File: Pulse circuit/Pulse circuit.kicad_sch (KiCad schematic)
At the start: 5 parts, among them U1 module_max30102, U2 module_max30102, U3 DOIT-ESP32-DEVKIT-V1

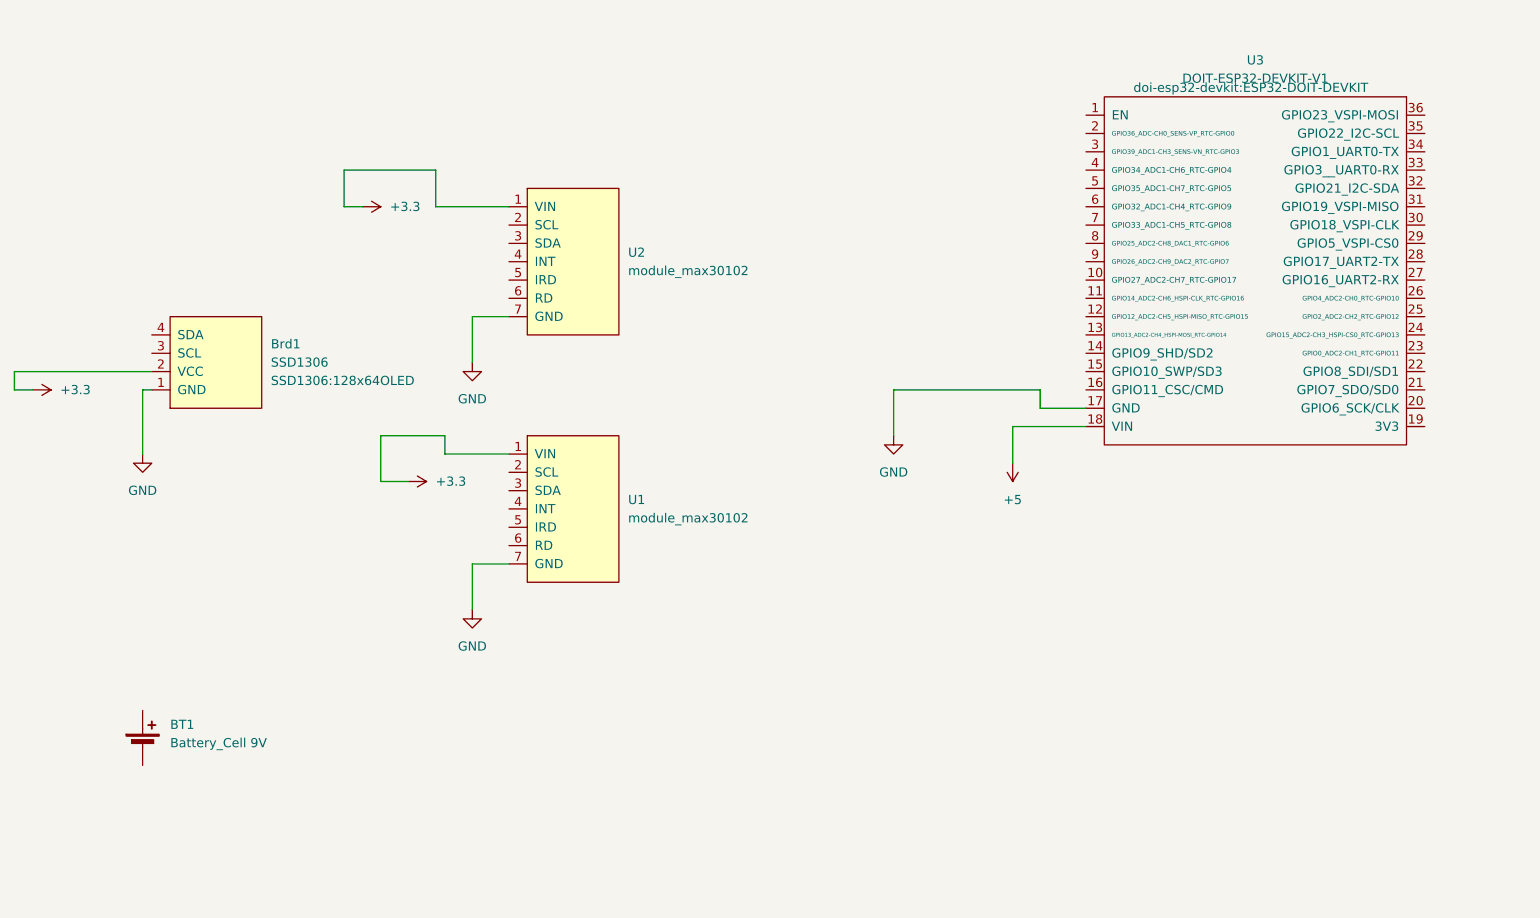
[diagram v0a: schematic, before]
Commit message: Not finished yet [Will do a revision tomorrow]
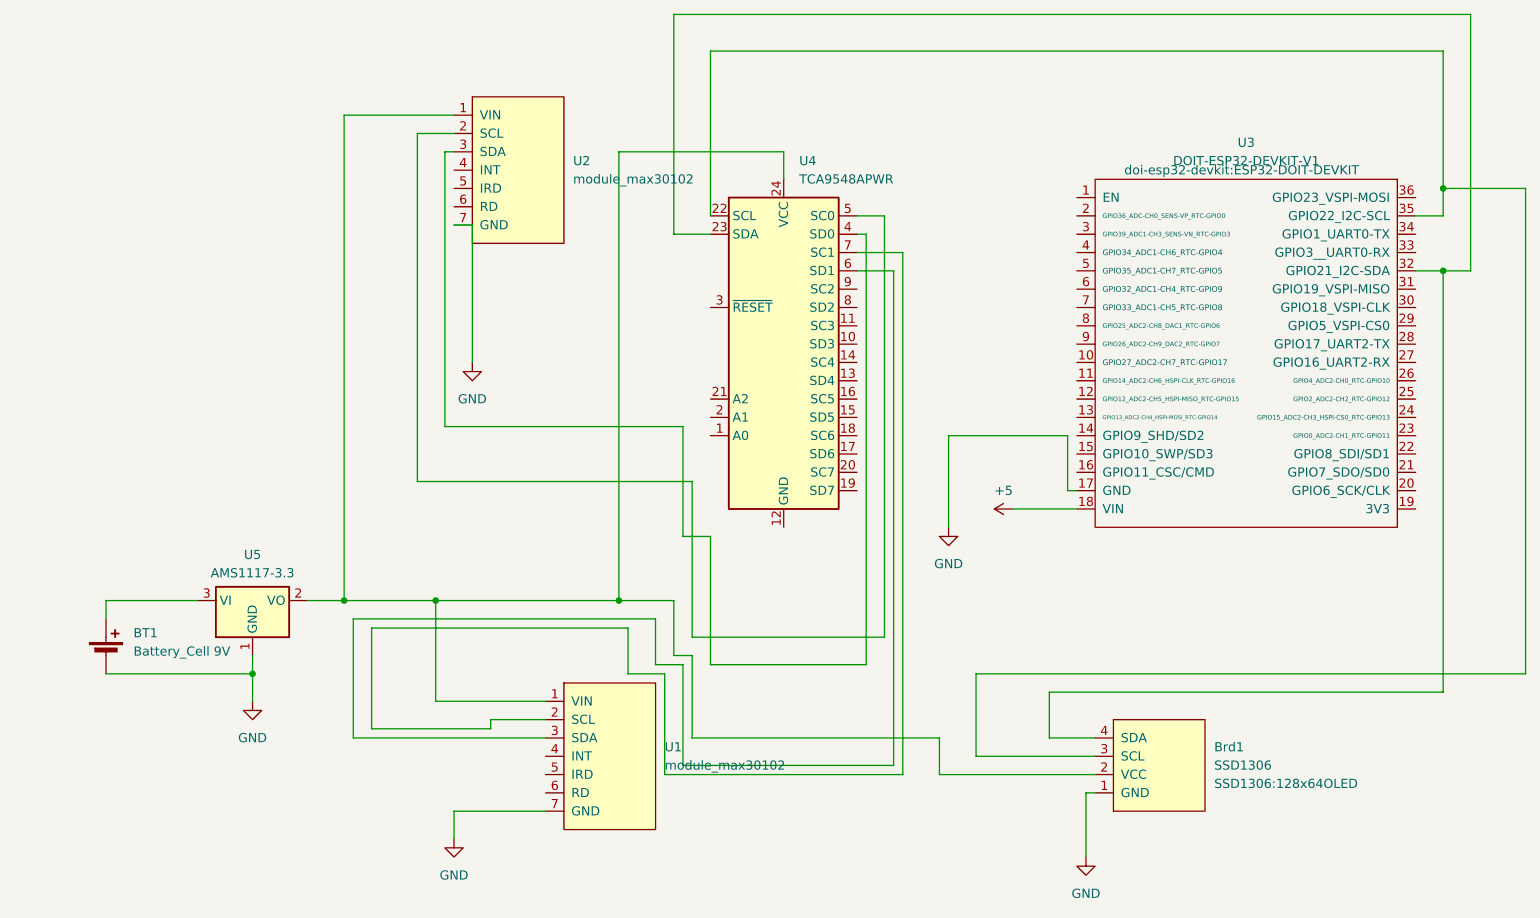
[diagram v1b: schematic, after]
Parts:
- added U4: TCA9548APWR, Package_SO:TSSOP-24_4.4x7.8mm_P0.65mm, symbol Interface_Expansion:TCA9548APWR
- added U5: AMS1117-3.3, Package_TO_SOT_SMD:SOT-223-3_TabPin2, symbol Regulator_Linear:AMS1117-3.3
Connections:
- net GND: now also BT1.2 (-), U5.1 (GND)
- net at BT1.1 (+): now also U5.3 (VI)
- net at U1.2 (SCL): now also U4.7 (SC1)
- net at U1.3 (SDA): now also U4.6 (SD1)
- net at U2.2 (SCL): now also U4.5 (SC0)
- net at U2.3 (SDA): now also U4.4 (SD0)
- net at U3.32 (GPIO21_I2C-SDA): now also Brd1.4 (SDA), U4.23 (SDA)
- net at U3.35 (GPIO22_I2C-SCL): now also Brd1.3 (SCL), U4.22 (SCL)
- net +3.3: no longer names the net of Brd1.2 (VCC), U1.1 (VIN), U2.1 (VIN)
- net +3.3: now also U4.24 (VCC), U5.2 (VO)
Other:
- moved on the sheet: BT1, Brd1, U1, U2, U3
